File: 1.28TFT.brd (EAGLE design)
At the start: 12 parts, among them M1 LCD_FPCST

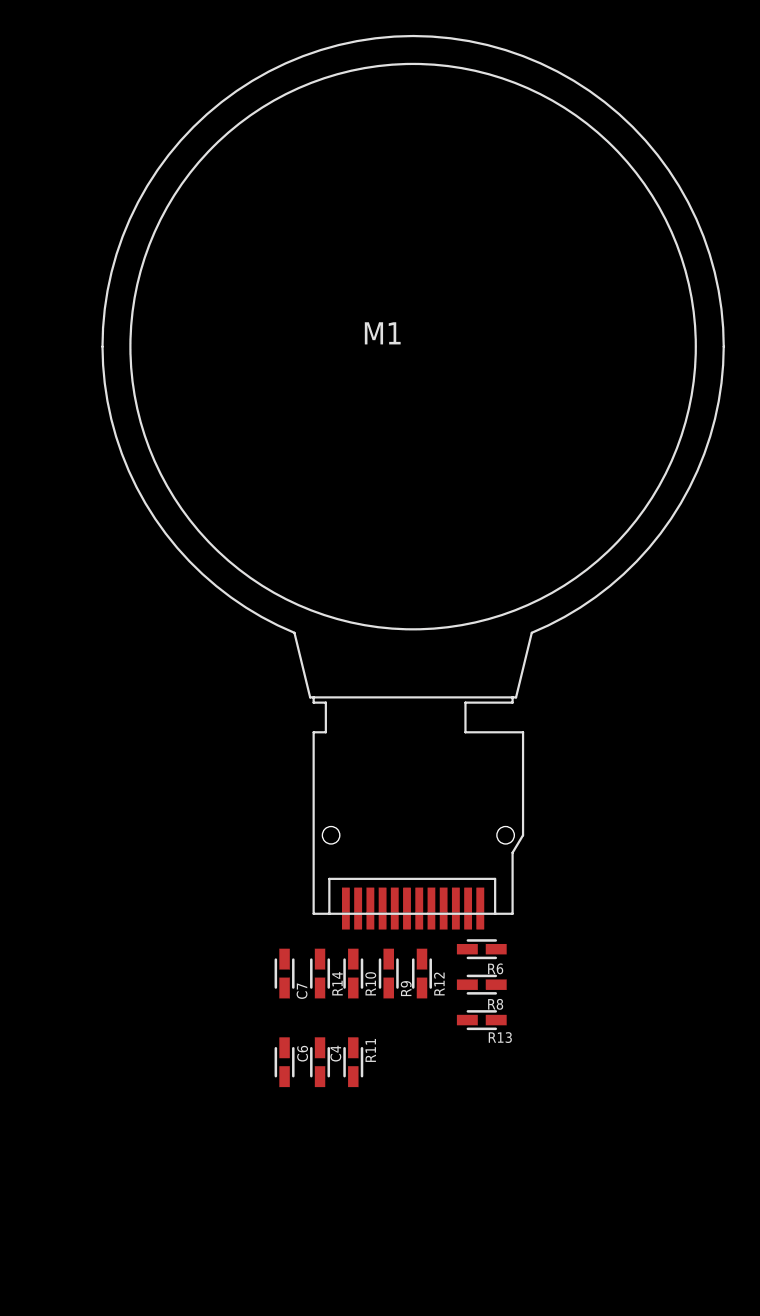
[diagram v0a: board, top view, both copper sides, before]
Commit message: design block
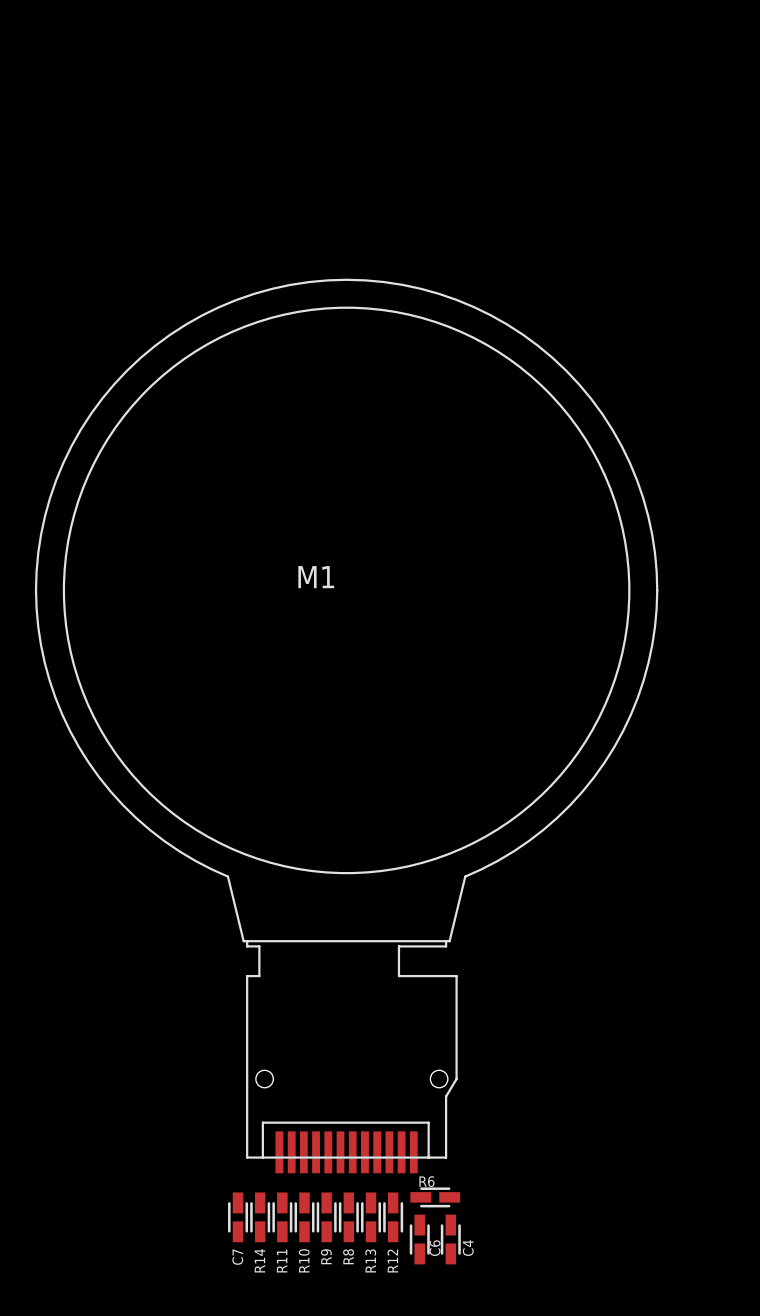
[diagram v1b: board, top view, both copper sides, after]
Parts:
- moved R8 15.4 mm to (7.24, 3.30), turned to 90 degrees
- moved M1 14.5 mm to (7.11, 38.6)
- moved R6 14.5 mm to (12.2, 4.45)
- moved R9 14.4 mm to (5.97, 3.30)
- moved R14 14.4 mm to (2.16, 3.30)
- moved R10 14.2 mm to (4.70, 3.30)
- moved C7 14.2 mm to (0.89, 3.30)
- moved R12 14.1 mm to (9.78, 3.30)
- moved R13 13.0 mm to (8.51, 3.30), turned to 270 degrees
- moved C6 12.8 mm to (11.3, 2.03), turned to 270 degrees
- moved C4 12.6 mm to (13.1, 2.03), turned to 270 degrees
- moved R11 9.77 mm to (3.43, 3.30)
